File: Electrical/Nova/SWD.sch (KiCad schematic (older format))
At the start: 2 parts

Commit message: Added Barometer, Flash, SD, and Power Supply
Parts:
- J? (x2): symbol Nova_Microcontroller:Conn_01x06_Male -> Nova-rescue:Conn_01x06_Male-Nova_Microcontroller
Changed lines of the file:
@@
 $Descr A4 11693 8268
 encoding utf-8
-Sheet 9 9
+Sheet 9 13
 Title "Microcontroller"
 Date "2020-07-02"
@@
 $EndDescr
 $Comp
-L Nova_Microcontroller:Conn_01x06_Male J?
+L Nova-rescue:Conn_01x06_Male-Nova_Microcontroller J?
 U 1 1 5F3A5F38
 P 5150 3600
@@
 $EndBitmap
 $Comp
-L Nova_Microcontroller:Conn_01x06_Male J?
+L Nova-rescue:Conn_01x06_Male-Nova_Microcontroller J?
 U 1 1 5EF13F12
 P 5150 3600

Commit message: Fixed Power Supply
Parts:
- J? (x2): symbol Nova-rescue:Conn_01x06_Male-Nova_Microcontroller -> Nova-rescue:Conn_01x06_Male-Nova_Microcontroller-Nova-rescue
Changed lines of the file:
@@
 $EndDescr
 $Comp
-L Nova-rescue:Conn_01x06_Male-Nova_Microcontroller J?
+L Nova-rescue:Conn_01x06_Male-Nova_Microcontroller-Nova-rescue J?
 U 1 1 5F3A5F38
 P 5150 3600
@@
 $EndBitmap
 $Comp
-L Nova-rescue:Conn_01x06_Male-Nova_Microcontroller J?
+L Nova-rescue:Conn_01x06_Male-Nova_Microcontroller-Nova-rescue J?
 U 1 1 5EF13F12
 P 5150 3600

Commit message: Added Gyroscope
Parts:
- J? (x2): symbol Nova-rescue:Conn_01x06_Male-Nova_Microcontroller-Nova-rescue -> Nova-rescue:Conn_01x06_Male-Nova_Microcontroller-Nova-rescue-Nova-rescue
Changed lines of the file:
@@
 $Descr A4 11693 8268
 encoding utf-8
-Sheet 9 13
+Sheet 9 14
 Title "Microcontroller"
 Date "2020-07-02"
@@
 $EndDescr
 $Comp
-L Nova-rescue:Conn_01x06_Male-Nova_Microcontroller-Nova-rescue J?
+L Nova-rescue:Conn_01x06_Male-Nova_Microcontroller-Nova-rescue-Nova-rescue J?
 U 1 1 5F3A5F38
 P 5150 3600
@@
 $EndBitmap
 $Comp
-L Nova-rescue:Conn_01x06_Male-Nova_Microcontroller-Nova-rescue J?
+L Nova-rescue:Conn_01x06_Male-Nova_Microcontroller-Nova-rescue-Nova-rescue J?
 U 1 1 5EF13F12
 P 5150 3600

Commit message: Added Gyro pins. Organized Schematic
Need to determine if we need the interrupt pins for the sensors.
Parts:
- J? (x2): symbol Nova-rescue:Conn_01x06_Male-Nova_Microcontroller-Nova-rescue-Nova-rescue -> Nova-rescue:Conn_01x06_Male-Nova_Microcontroller-Nova-rescue-Nova-rescue-Nova-rescue
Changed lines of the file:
@@
 $EndDescr
 $Comp
-L Nova-rescue:Conn_01x06_Male-Nova_Microcontroller-Nova-rescue-Nova-rescue J?
+L Nova-rescue:Conn_01x06_Male-Nova_Microcontroller-Nova-rescue-Nova-rescue-Nova-rescue J?
 U 1 1 5F3A5F38
 P 5150 3600
@@
 $EndBitmap
 $Comp
-L Nova-rescue:Conn_01x06_Male-Nova_Microcontroller-Nova-rescue-Nova-rescue J?
+L Nova-rescue:Conn_01x06_Male-Nova_Microcontroller-Nova-rescue-Nova-rescue-Nova-rescue J?
 U 1 1 5EF13F12
 P 5150 3600

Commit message: Added Pyro Channels
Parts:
- J? (x2): symbol Nova-rescue:Conn_01x06_Male-Nova_Microcontroller-Nova-rescue-Nova-rescue-Nova-rescue -> Nova-rescue:Conn_01x06_Male-Nova_Microcontroller-Nova-rescue-Nova-rescue-Nova-rescue-Nova-rescue
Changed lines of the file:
@@
 $Descr A4 11693 8268
 encoding utf-8
-Sheet 9 14
+Sheet 9 16
 Title "Microcontroller"
 Date "2020-07-02"
@@
 $EndDescr
 $Comp
-L Nova-rescue:Conn_01x06_Male-Nova_Microcontroller-Nova-rescue-Nova-rescue-Nova-rescue J?
+L Nova-rescue:Conn_01x06_Male-Nova_Microcontroller-Nova-rescue-Nova-rescue-Nova-rescue-Nova-rescue J?
 U 1 1 5F3A5F38
 P 5150 3600
@@
 $EndBitmap
 $Comp
-L Nova-rescue:Conn_01x06_Male-Nova_Microcontroller-Nova-rescue-Nova-rescue-Nova-rescue J?
+L Nova-rescue:Conn_01x06_Male-Nova_Microcontroller-Nova-rescue-Nova-rescue-Nova-rescue-Nova-rescue J?
 U 1 1 5EF13F12
 P 5150 3600

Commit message: Added LED sheet and pins
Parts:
- J? (x2): symbol Nova-rescue:Conn_01x06_Male-Nova_Microcontroller-Nova-rescue-Nova-rescue-Nova-rescue-Nova-rescue -> Nova-rescue:Conn_01x06_Male-Nova_Microcontroller-Nova-rescue-Nova-rescue-Nova-rescue-Nova-rescue-Nova-rescue
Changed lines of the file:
@@
 $Descr A4 11693 8268
 encoding utf-8
-Sheet 9 16
+Sheet 9 18
 Title "Microcontroller"
 Date "2020-07-02"
@@
 $EndDescr
 $Comp
-L Nova-rescue:Conn_01x06_Male-Nova_Microcontroller-Nova-rescue-Nova-rescue-Nova-rescue-Nova-rescue J?
+L Nova-rescue:Conn_01x06_Male-Nova_Microcontroller-Nova-rescue-Nova-rescue-Nova-rescue-Nova-rescue-Nova-rescue J?
 U 1 1 5F3A5F38
 P 5150 3600
@@
 $EndBitmap
 $Comp
-L Nova-rescue:Conn_01x06_Male-Nova_Microcontroller-Nova-rescue-Nova-rescue-Nova-rescue-Nova-rescue J?
+L Nova-rescue:Conn_01x06_Male-Nova_Microcontroller-Nova-rescue-Nova-rescue-Nova-rescue-Nova-rescue-Nova-rescue J?
 U 1 1 5EF13F12
 P 5150 3600

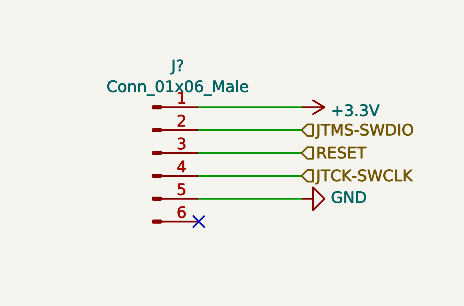
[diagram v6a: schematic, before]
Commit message: Minor update
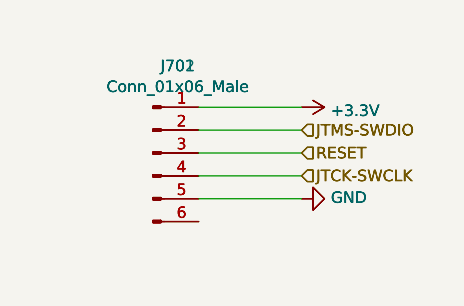
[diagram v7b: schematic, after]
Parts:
- gave numbers to parts that had none: 2
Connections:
- no-connect marks 2 -> 0
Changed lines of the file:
@@
 $Descr A4 11693 8268
 encoding utf-8
-Sheet 9 18
+Sheet 7 18
 Title "Microcontroller"
 Date "2020-07-02"
@@
 $EndDescr
 $Comp
-L Nova-rescue:Conn_01x06_Male-Nova_Microcontroller-Nova-rescue-Nova-rescue-Nova-rescue-Nova-rescue-Nova-rescue J?
+L Nova-rescue:Conn_01x06_Male-Nova_Microcontroller-Nova-rescue-Nova-rescue-Nova-rescue-Nova-rescue-Nova-rescue J702
 U 1 1 5F3A5F38
 P 5150 3600
-F 0 "J?" H 5258 3981 50  0000 C CNN
+F 0 "J702" H 5258 3981 50  0000 C CNN
 F 1 "Conn_01x06_Male" H 5258 3890 50  0000 C CNN
 F 2 "NOVA MCU (STM):j-link_6_pin_needle" H 5150 3600 50  0001 C CNN
@@
 $EndComp
 $Comp
-L power:+3.3V #PWR?
+L power:+3.3V #PWR0702
 U 1 1 5F3A5F39
 P 5800 3400
-F 0 "#PWR?" H 5800 3250 50  0001 C CNN
+F 0 "#PWR0702" H 5800 3250 50  0001 C CNN
 F 1 "+3.3V" V 5815 3528 50  0000 L CNN
 F 2 "" H 5800 3400 50  0001 C CNN
@@
 $EndComp
 $Comp
-L power:GND #PWR?
+L power:GND #PWR0703
 U 1 1 5EF14A6C
 P 5800 3800
-F 0 "#PWR?" H 5800 3550 50  0001 C CNN
+F 0 "#PWR0703" H 5800 3550 50  0001 C CNN
 F 1 "GND" V 5805 3672 50  0000 R CNN
 F 2 "" H 5800 3800 50  0001 C CNN
@@
 Wire Wire Line
 	5350 3600 5800 3600
-NoConn ~ 5350 3900
 Text HLabel 5800 3600 2    50   Input ~ 0
 RESET
@@
 $EndBitmap
 $Comp
-L Nova-rescue:Conn_01x06_Male-Nova_Microcontroller-Nova-rescue-Nova-rescue-Nova-rescue-Nova-rescue-Nova-rescue J?
+L Nova-rescue:Conn_01x06_Male-Nova_Microcontroller-Nova-rescue-Nova-rescue-Nova-rescue-Nova-rescue-Nova-rescue J701
 U 1 1 5EF13F12
 P 5150 3600
-F 0 "J?" H 5258 3981 50  0000 C CNN
+F 0 "J701" H 5258 3981 50  0000 C CNN
 F 1 "Conn_01x06_Male" H 5258 3890 50  0000 C CNN
 F 2 "NOVA MCU (STM):j-link_6_pin_needle" H 5150 3600 50  0001 C CNN
@@
 $EndComp
 $Comp
-L power:+3.3V #PWR?
+L power:+3.3V #PWR0701
 U 1 1 5EF1469E
 P 5800 3400
-F 0 "#PWR?" H 5800 3250 50  0001 C CNN
+F 0 "#PWR0701" H 5800 3250 50  0001 C CNN
 F 1 "+3.3V" V 5815 3528 50  0000 L CNN
 F 2 "" H 5800 3400 50  0001 C CNN
@@
 $EndComp
 $Comp
-L power:GND #PWR?
+L power:GND #PWR0704
 U 1 1 5F3A5F3A
 P 5800 3800
-F 0 "#PWR?" H 5800 3550 50  0001 C CNN
+F 0 "#PWR0704" H 5800 3550 50  0001 C CNN
 F 1 "GND" V 5805 3672 50  0000 R CNN
 F 2 "" H 5800 3800 50  0001 C CNN
@@
 	0    -1   -1   0
 $EndComp
-Wire Wire Line
-	5350 3400 5800 3400
-Wire Wire Line
-	5350 3800 5800 3800
 Text HLabel 5800 3500 2    50   Input ~ 0
 JTMS-SWDIO
 Text HLabel 5800 3700 2    50   Input ~ 0
 JTCK-SWCLK
-Wire Wire Line
-	5350 3500 5800 3500
-Wire Wire Line
-	5350 3600 5800 3600
-NoConn ~ 5350 3900
 Text HLabel 5800 3600 2    50   Input ~ 0
 RESET
-Wire Wire Line
-	5350 3700 5800 3700
 $Bitmap
 Pos 9100 7700

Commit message: Added Accelerometer
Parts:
- J701, J702: symbol Nova-rescue:Conn_01x06_Male-Nova_Microcontroller-Nova-rescue-Nova-rescue-Nova-rescue-Nova-rescue-Nova-rescue -> Nova-rescue:Conn_01x06_Male-Nova_Microcontroller-Nova-rescue-Nova-rescue-Nova-rescue-Nova-rescue-Nova-rescue-Nova-rescue
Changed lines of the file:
@@
 $Descr A4 11693 8268
 encoding utf-8
-Sheet 7 18
+Sheet 7 19
 Title "Microcontroller"
 Date "2020-07-02"
@@
 $EndDescr
 $Comp
-L Nova-rescue:Conn_01x06_Male-Nova_Microcontroller-Nova-rescue-Nova-rescue-Nova-rescue-Nova-rescue-Nova-rescue J702
+L Nova-rescue:Conn_01x06_Male-Nova_Microcontroller-Nova-rescue-Nova-rescue-Nova-rescue-Nova-rescue-Nova-rescue-Nova-rescue J702
 U 1 1 5F3A5F38
 P 5150 3600
@@
 $EndBitmap
 $Comp
-L Nova-rescue:Conn_01x06_Male-Nova_Microcontroller-Nova-rescue-Nova-rescue-Nova-rescue-Nova-rescue-Nova-rescue J701
+L Nova-rescue:Conn_01x06_Male-Nova_Microcontroller-Nova-rescue-Nova-rescue-Nova-rescue-Nova-rescue-Nova-rescue-Nova-rescue J701
 U 1 1 5EF13F12
 P 5150 3600
